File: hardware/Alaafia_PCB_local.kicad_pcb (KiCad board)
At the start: 2 copper layers, 69.5 x 48.6 mm, 6 parts, among them J1 BATTERY, U1 ESP32-C3_SUPERMINI, U2 BMI160, U3 MT3608

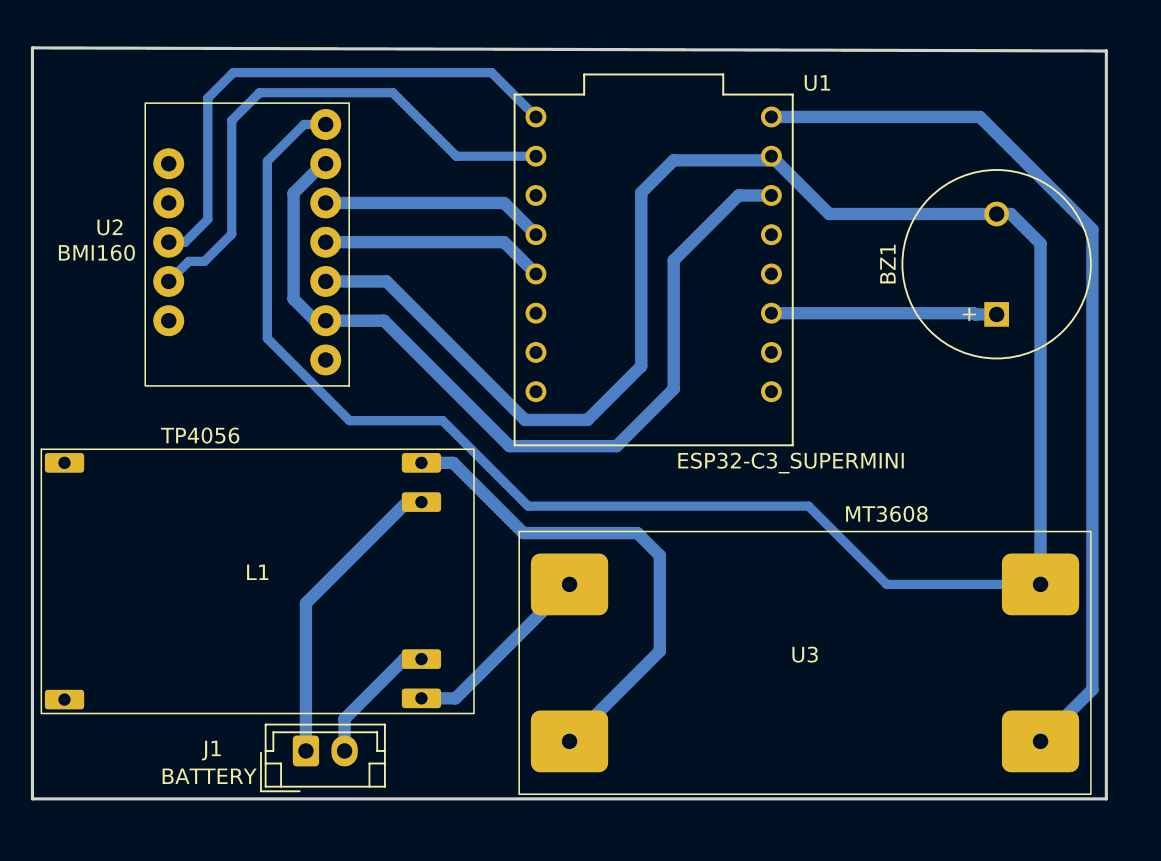
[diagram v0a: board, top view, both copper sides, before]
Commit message: Before pulling idf framework
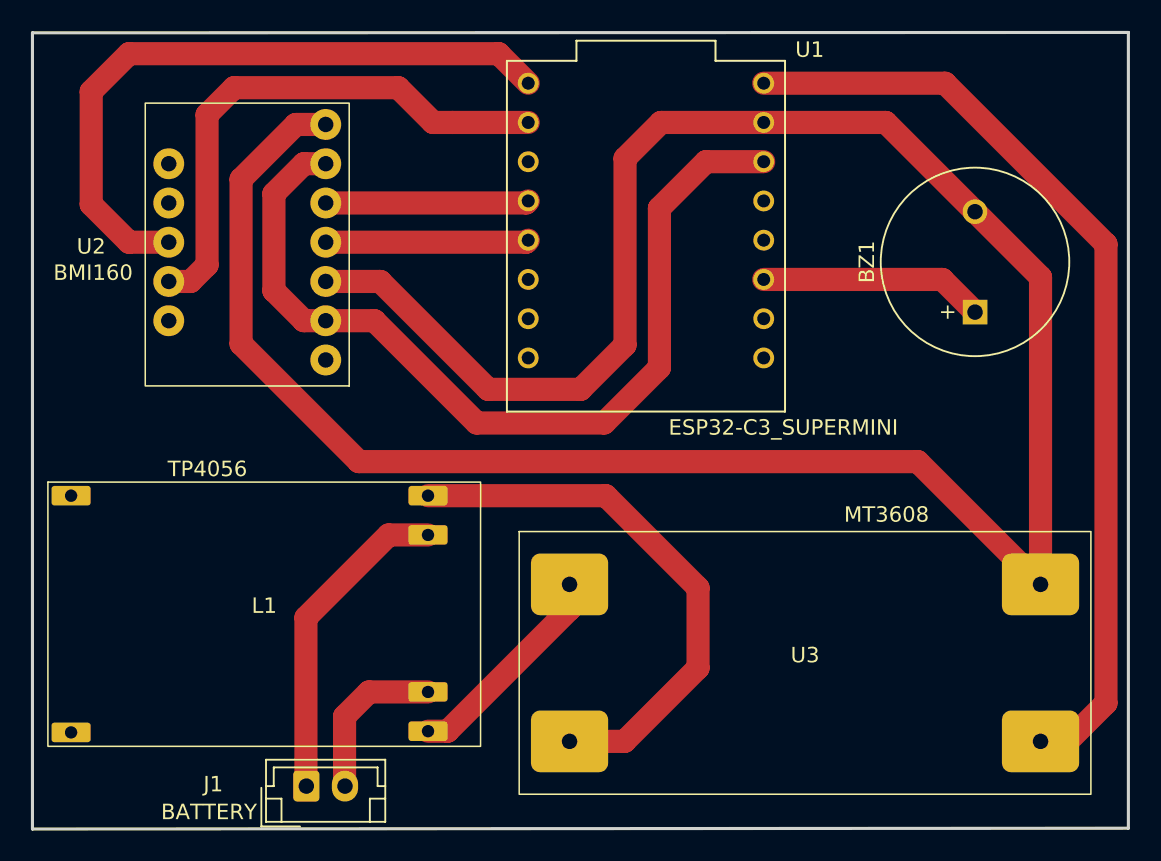
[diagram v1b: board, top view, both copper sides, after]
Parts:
- moved J1 2.28 mm to (131.2, 103.5)
- moved U1 2.24 mm to (153.2, 67.9)
- moved L1 2.17 mm to (128.5, 92.3)
- moved BZ1 1.41 mm to (174.5, 72.8)
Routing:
- net /INT1: track 34.1 -> 43.4 mm
- net /5V: track 58.3 -> 61.4 mm
- net Net-(L1-OUT+): track 32.4 -> 35.4 mm
- net /3V3: track 56.2 -> 58.7 mm
- net /GND: track 160.9 -> 163.2 mm
- net Net-(L1-B-): track 8.65 -> 10.6 mm
- net Net-(L1-OUT-): track 12.6 -> 14.0 mm
- net /SDA: track 14.5 -> 13.2 mm
- net /SCL: track 14.5 -> 13.2 mm
- net Net-(L1-B+): track 19.7 -> 21.0 mm
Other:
- board size 69.5 x 48.6 mm -> 70.9 x 51.5 mm
